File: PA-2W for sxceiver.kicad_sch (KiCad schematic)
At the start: 40 parts, among them J1 SMA_RF IN, J2 SMA_RF OUT, J3 5Vcc input, U1 TQP3M9036, U3 TQP7M9106

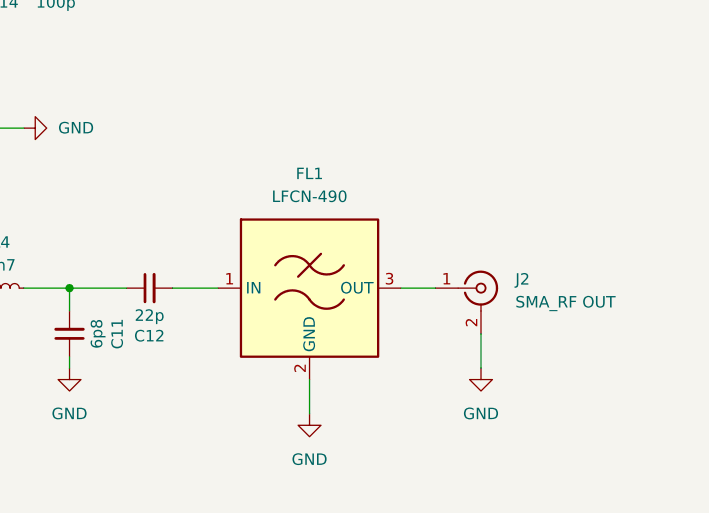
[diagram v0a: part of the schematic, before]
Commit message: Add files via upload
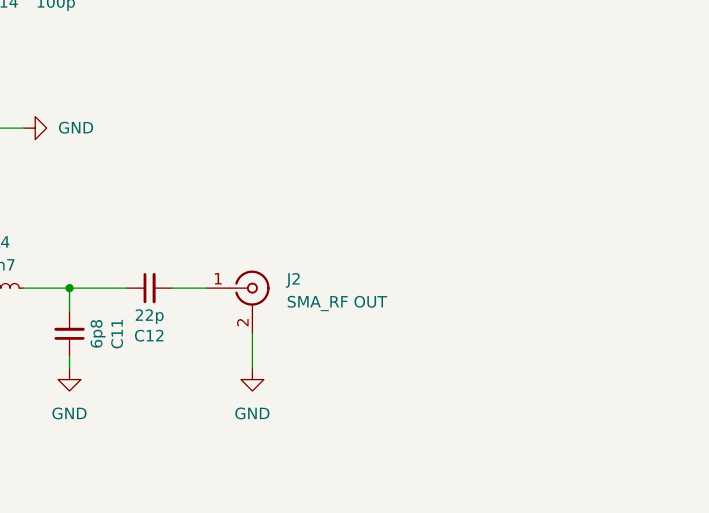
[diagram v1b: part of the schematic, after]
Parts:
- removed FL1: LFCN-490, Filter:Filter_Mini-Circuits_FV1206, symbol RF_Filter:LFCN-490
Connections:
- net at C12.2: now also J2.1 (In)
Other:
- moved on the sheet: J2
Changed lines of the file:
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@@
 	(title_block
 		(title "SXceiver High Linearity Amplifier up to 2W")
-		(date "2026-03-15")
-		(rev "V1.0")
+		(date "2026-03-21")
+		(rev "V1.1")
 		(company "Z32IT")
 	)
@@
 	(wire
 		(pts
-			(xy 224.79 114.3) (xy 229.87 114.3)
-		)
-		(stroke
-			(width 0)
-			(type default)
-		)
-	)
-	(wire
-		(pts
 			(xy 74.93 55.88) (xy 90.17 55.88)
 		)
@@
 	(wire
 		(pts
-			(xy 250.19 114.3) (xy 254 114.3)
+			(xy 224.79 114.3) (xy 228.6 114.3)
 		)
 		(stroke
@@
 	(wire
 		(pts
-			(xy 259.08 119.38) (xy 259.08 123.19)
+			(xy 233.68 119.38) (xy 233.68 123.19)
 		)
 		(stroke
@@
 	(wire
 		(pts
-			(xy 240.03 124.46) (xy 240.03 128.27)
-		)
-		(stroke
-			(width 0)
-			(type default)
-		)
-	)
-	(wire
-		(pts
 			(xy 68.58 55.88) (xy 74.93 55.88)
 		)
@@
 	)
 	(symbol
-		(lib_id "PCM_4ms_Power-symbol:GND")
-		(at 240.03 128.27 0)
-		(unit 1)
-		(exclude_from_sim no)
-		(in_bom yes)
-		(on_board yes)
-		(dnp no)
-		(fields_autoplaced yes)
-		(property "Reference" "#PWR013"
-			(at 240.03 134.62 0)
-			(effects
-				(font
-					(size 1.27 1.27)
-				)
-				(hide yes)
-			)
-		)
-		(property "Value" "GND"
-			(at 240.03 133.35 0)
-			(effects
-				(font
-					(size 1.27 1.27)
-				)
-			)
-		)
-		(property "Footprint" ""
-			(at 240.03 128.27 0)
-			(effects
-				(font
-					(size 1.27 1.27)
-				)
-				(hide yes)
-			)
-		)
-		(property "Datasheet" ""
-			(at 240.03 128.27 0)
-			(effects
-				(font
-					(size 1.27 1.27)
-				)
-				(hide yes)
-			)
-		)
-		(property "Description" ""
-			(at 240.03 128.27 0)
-			(effects
-				(font
-					(size 1.27 1.27)
-				)
-				(hide yes)
-			)
-		)
-		(pin "1"
-		)
-		(instances
-			(project "LNA-2W"
-				(path "/9e841ece-bd19-4cb2-9a9c-7f7db9f00b2a"
-					(reference "#PWR013")
-					(unit 1)
-				)
-			)
-		)
-	)
-	(symbol
 		(lib_id "power:GND")
 		(at 80.01 71.12 0)
@@
 	)
 	(symbol
-		(lib_id "RF_Filter:LFCN-490")
-		(at 240.03 114.3 0)
-		(unit 1)
-		(exclude_from_sim no)
-		(in_bom yes)
-		(on_board yes)
-		(dnp no)
-		(fields_autoplaced yes)
-		(property "Reference" "FL1"
-			(at 240.03 101.6 0)
-			(effects
-				(font
-					(size 1.27 1.27)
-				)
-			)
-		)
-		(property "Value" "LFCN-490"
-			(at 240.03 104.14 0)
-			(effects
-				(font
-					(size 1.27 1.27)
-				)
-			)
-		)
-		(property "Footprint" "Filter:Filter_Mini-Circuits_FV1206"
-			(at 240.03 101.6 0)
-			(effects
-				(font
-					(size 1.27 1.27)
-				)
-				(hide yes)
-			)
-		)
-		(property "Datasheet" "https://www.minicircuits.com/pdfs/LFCN-490+.pdf"
-			(at 240.03 114.3 0)
-			(effects
-				(font
-					(size 1.27 1.27)
-				)
-				(hide yes)
-			)
-		)
-		(property "Description" "490MHz 50 Ohm Passive Low Pass Filter, FV1206"
-			(at 240.03 114.3 0)
-			(effects
-				(font
-					(size 1.27 1.27)
-				)
-				(hide yes)
-			)
-		)
-		(pin "1"
-		)
-		(pin "2"
-		)
-		(pin "3"
-		)
-		(pin "4"
-		)
-		(instances
-			(project ""
-				(path "/9e841ece-bd19-4cb2-9a9c-7f7db9f00b2a"
-					(reference "FL1")
-					(unit 1)
-				)
-			)
-		)
-	)
-	(symbol
 		(lib_id "Mechanical:MountingHole")
 		(at 264.16 26.67 0)
@@
 	(symbol
 		(lib_id "Connector:Conn_Coaxial")
-		(at 259.08 114.3 0)
+		(at 233.68 114.3 0)
 		(unit 1)
 		(exclude_from_sim no)
@@
 		(fields_autoplaced yes)
 		(property "Reference" "J2"
-			(at 262.89 113.3231 0)
+			(at 237.49 113.3231 0)
 			(effects
 				(font
@@
 		)
 		(property "Value" "SMA_RF OUT"
-			(at 262.89 115.8631 0)
+			(at 237.49 115.8631 0)
 			(effects
 				(font
@@
 		)
 		(property "Footprint" "PCM_SparkFun-Connector:SMA_Edge_6.3mm"
-			(at 259.08 114.3 0)
+			(at 233.68 114.3 0)
 			(effects
 				(font
@@
 		)
 		(property "Datasheet" "~"
-			(at 259.08 114.3 0)
+			(at 233.68 114.3 0)
 			(effects
 				(font
@@
 		)
 		(property "Description" "coaxial connector (BNC, SMA, SMB, SMC, Cinch/RCA, LEMO, ...)"
-			(at 259.08 114.3 0)
+			(at 233.68 114.3 0)
 			(effects
 				(font
@@
 	(symbol
 		(lib_id "PCM_4ms_Power-symbol:GND")
-		(at 259.08 123.19 0)
+		(at 233.68 123.19 0)
 		(unit 1)
 		(exclude_from_sim no)
@@
 		(fields_autoplaced yes)
 		(property "Reference" "#PWR04"
-			(at 259.08 129.54 0)
+			(at 233.68 129.54 0)
 			(effects
 				(font
@@
 		)
 		(property "Value" "GND"
-			(at 259.08 128.27 0)
+			(at 233.68 128.27 0)
 			(effects
 				(font
@@
 		)
 		(property "Footprint" ""
-			(at 259.08 123.19 0)
+			(at 233.68 123.19 0)
 			(effects
 				(font
@@
 		)
 		(property "Datasheet" ""
-			(at 259.08 123.19 0)
+			(at 233.68 123.19 0)
 			(effects
 				(font
@@
 		)
 		(property "Description" ""
-			(at 259.08 123.19 0)
+			(at 233.68 123.19 0)
 			(effects
 				(font
